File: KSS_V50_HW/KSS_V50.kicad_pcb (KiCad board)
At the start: 4 copper layers, 159 x 21.7 mm, 128 parts, among them J1 Conn_01x02_Socket, J2 Conn_01x04_Socket, J3 Conn_01x04_Socket, J4 Conn_01x02_Socket, J5 Conn_01x04_Pin, J6 Conn_01x04_Pin, Q1 DMG3414U-7, Q2 DMG3414U-7, Q5 DMG3414U-7, Q6 SSM3J332R,LF, SW2 SW_SP3T, U1 SPV1040, U10 ATtiny3226-X, U11 AT42QT1010-TSHR, U12 SN74AUP1T34DCK, U13 SN74AUP1T34DCK, U14 SN74AUP1T34DCK, U15 SN74AUP1T34DCK, U2 INA236, U3 BQ29737, U4 INA236, U5 TPS62843, U6 TMAG5328, U7 TMC2300-LA-T, U8 TMAG5328, U9 TMC2300-LA-T

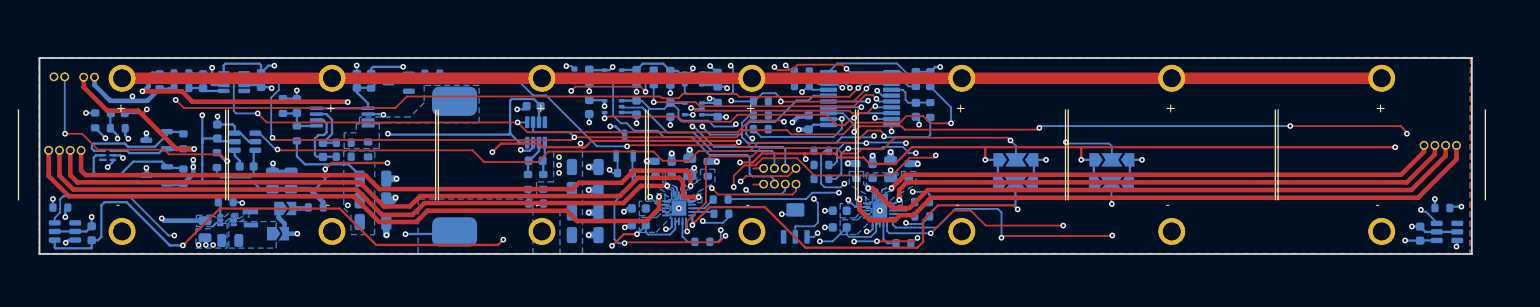
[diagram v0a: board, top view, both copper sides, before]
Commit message: post assembly commit
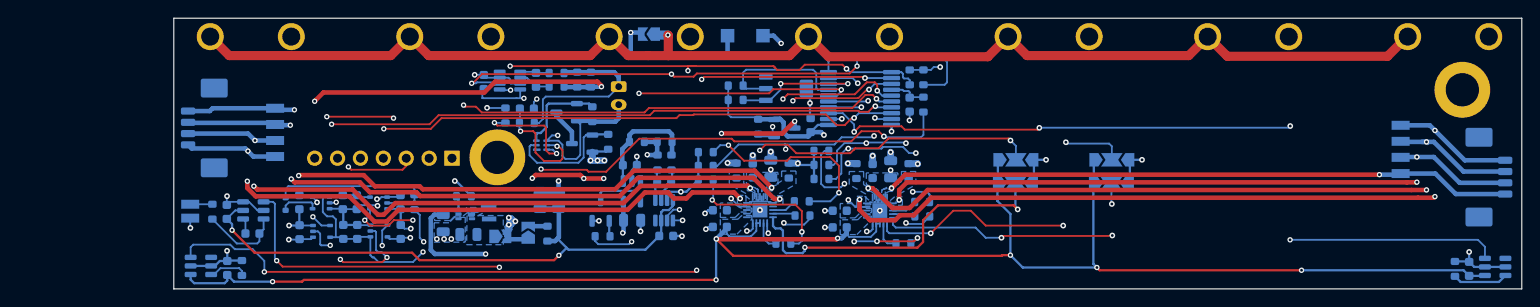
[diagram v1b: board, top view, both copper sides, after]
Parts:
- removed C1, C2, C3, C4, C7: 47 uF, Capacitor_SMD:C_1206_3216Metric
- removed C10: 1nF, Capacitor_SMD:C_0603_1608Metric
- removed C8: 1uF, Capacitor_SMD:C_0603_1608Metric
- removed C9: 100nF, Capacitor_SMD:C_0603_1608Metric
- removed J6: Conn_01x04_Pin, ap_built:Debug_Header
- removed L1: 47uH, ap_built:AMDLA1306Q-470MT
- removed R4, R6: 1k, Resistor_SMD:R_0603_1608Metric
- removed R5: 1Meg, Resistor_SMD:R_0603_1608Metric
- removed R7: 210k, Resistor_SMD:R_0603_1608Metric
- added H1: MountingHole, ap_built:24929, B.Cu at (122.0, 100.7)
- added H2: MountingHole, ap_built:24929, B.Cu at (229.1, 93.2)
- added J7: Conn_01x04_Socket, Connector_Molex:Molex_PicoBlade_53261-0471_1x04-1MP_P1.25mm_Horizontal, B.Cu at (90.0, 97.4)
- added J8: Conn_01x04_Socket, Connector_Molex:Molex_PicoBlade_53261-0471_1x04-1MP_P1.25mm_Horizontal, B.Cu at (231.4, 102.9)
- added JP6: SolderJumper_2_Bridged, Jumper:SolderJumper-2_P1.3mm_Open_TrianglePad1.0x1.5mm, B.Cu at (138.8, 87.0)
- added TP1: TestPoint, TestPoint:TestPoint_Pad_1.5x1.5mm, B.Cu at (147.5, 87.2)
- added TP2: TestPoint, TestPoint:TestPoint_Pad_1.5x1.5mm, B.Cu at (151.4, 87.2)
- C5: value 47 uF -> 10uF; footprint Capacitor_SMD:C_1206_3216Metric -> Capacitor_SMD:C_0805_2012Metric
- C6: value 47 uF -> 1uF; footprint Capacitor_SMD:C_1206_3216Metric -> Capacitor_SMD:C_0603_1608Metric
- J1: footprint ap_built:Batt_Header -> Connector_JST:JST_PH_S2B-PH-K_1x02_P2.00mm_Horizontal
- J5: value Conn_01x04_Pin -> Conn_01x07_Pin; footprint ap_built:Debug_Header -> Connector_PinHeader_2.54mm:PinHeader_1x07_P2.54mm_Horizontal
- L2: footprint Inductor_SMD:L_Murata_DFE201610P -> ap_built:L_Murata_DFE201610P
- R2: value 250m -> 0
- R3: value 1k -> 0
- SC1, SC2, SC3, SC4, SC5, SC6, SC7: footprint ap_built:SM141K04TFS -> ap_built:SM101K07L
- U1: value SPV1040 -> MAX40200AUK; footprint Package_SO:TSSOP-8_4.4x3mm_P0.65mm -> Package_TO_SOT_SMD:SOT-23-5
- U7, U9: footprint Package_DFN_QFN:QFN-20-1EP_3x3mm_P0.4mm_EP1.65x1.65mm -> ap_built:QFN-20-1EP_3x3mm_P0.4mm_EP1.65x1.65mm
- moved J1 60.0 mm to (135.4, 92.8), turned to -90 degrees
- moved C39 48.3 mm to (100.0, 109.0), turned to 90 degrees
- moved U3 48.2 mm to (126.8, 99.3)
- moved Q2 47.3 mm to (131.4, 99.2)
- moved R14 47.3 mm to (134.2, 99.0)
- moved R10 46.3 mm to (130.8, 92.0), turned to -90 degrees
- moved Q1 45.6 mm to (129.6, 95.7)
- moved R12 45.5 mm to (122.8, 96.0)
- moved R13 45.5 mm to (132.5, 95.9)
- moved R11 45.4 mm to (125.2, 96.8)
- moved C13 45.4 mm to (125.2, 95.3)
- moved U14 43.4 mm to (102.4, 108.9), turned to 0 degrees
- moved R15 41.7 mm to (128.5, 91.3), turned to 180 degrees
- moved R16 41.7 mm to (128.5, 92.8), turned to 180 degrees
- moved C38 38.7 mm to (104.9, 109.0), turned to 90 degrees
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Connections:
- C16 pad 1: /2_5V_Buck_Boost/VBAT_POS -> +V_BAT
- C38 pad 1: +V_COMM_EXT -> +V_PROG_EXT
- C40 pad 1: +V_COMM_EXT -> +V_PROG_EXT
- C5 pad 1: /2_5V_Buck_Boost/VBAT_POS -> +V_BAT
- C6 pad 1: /2_5V_Buck_Boost/VBAT_POS -> Net-(U1-VDD)
- J5 pad 4: GND -> /MCU_Prog_Comm/RX_COMM_EXT
- R1 pad 1: /MPPT/Solar_Cell_Out -> Net-(JP6-B)
- R1 pad 2: Net-(L1-Pad1) -> Net-(U1-VDD)
- R10 pad 2: /2_5V_Buck_Boost/VBAT_POS -> +V_BAT
- R16 pad 1: /2_5V_Buck_Boost/VBAT_POS -> +V_BAT
- R2 pad 1: Net-(U1-VOUT) -> Net-(U1-VDD)
- R2 pad 2: /2_5V_Buck_Boost/VBAT_POS -> Net-(JP6-B)
- R3 pad 1: Net-(U1-ICTRL_PLUS) -> +V_BAT
- R3 pad 2: Net-(U1-VOUT) -> Net-(J1-Pin_1)
- R8 pad 1: /MPPT/Solar_Cell_Out -> Net-(JP6-B)
- R9 pad 1: Net-(L1-Pad1) -> Net-(U1-VDD)
- U1 pad 1: Net-(Q5-D) -> Net-(U1-VDD)
- U1 pad 3: Net-(U1-Lx) -> Net-(Q5-D)
- U1 pad 4: Net-(U1-VOUT) -> unconnected-(U1-NC-Pad4)
- U1 pad 5: Net-(U1-VCTRL) -> +V_BAT
- U14 pad 5: +V_COMM_EXT -> +V_PROG_EXT
- U15 pad 1: +V_COMM_EXT -> +V_PROG_EXT
- U5 pad 2: /2_5V_Buck_Boost/VBAT_POS -> +V_BAT
- U5 pad 4: /2_5V_Buck_Boost/VBAT_POS -> +V_BAT
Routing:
- net +V_BAT: track 0.00 -> 97.6 mm, vias 0 -> 7
- net /2_5V_Buck_Boost/VBAT_POS: track 70.0 -> 0.00 mm, vias 4 -> 0
- net /MCU/MCU_TX: track 24.1 -> 80.1 mm, vias 2 -> 3
- net /MCU/MOT_STBY: track 69.5 -> 20.4 mm, vias 5 -> 3
- net /MCU/MCU_UPDI: track 29.3 -> 70.1 mm, vias 2 -> 3
- net /MCU/MCU_RX: track 34.2 -> 74.5 mm, vias 2 -> 3
- net Net-(JP6-B): track 0.00 -> 35.4 mm, vias 0 -> 2
- net +V_COMM_EXT: track 30.3 -> 0.00 mm, vias 2 -> 0
- net Net-(L1-Pad1): track 30.0 -> 0.00 mm, vias 2 -> 0
- net /SDA: track 111.7 -> 84.8 mm, vias 3 -> 4
- net /VIO_MOT: track 251.9 -> 225.1 mm, vias 15 -> 9
- net Net-(J4-Pin_1): track 27.1 -> 2.46 mm, vias 2 -> 0
- net /SCL: track 93.3 -> 69.6 mm
- net /Motor_Driver_2/OB2: track 72.2 -> 87.1 mm, vias 1 -> 3
- net /MCU_Prog_Comm/TX_PROG_EXT: track 27.5 -> 12.8 mm, vias 0 -> 2
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- added copper zone on B.Cu, net +V_BAT
- removed copper zone on B.Cu, net /2_5V_Buck_Boost/VBAT_POS
- removed copper zone on B.Cu, net /MPPT/Solar_Cell_Out
- removed copper zone on F.Cu, net GND
- removed copper zone on B.Cu, net Net-(L1-Pad1)
- removed copper zone on B.Cu, net Net-(U1-Lx)
- removed copper zone on B.Cu, net Net-(U1-VOUT)
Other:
- board size 159 x 21.7 mm -> 149.6 x 30 mm
